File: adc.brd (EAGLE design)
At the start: 20 parts, among them U1 LM4562MAX/NOPB

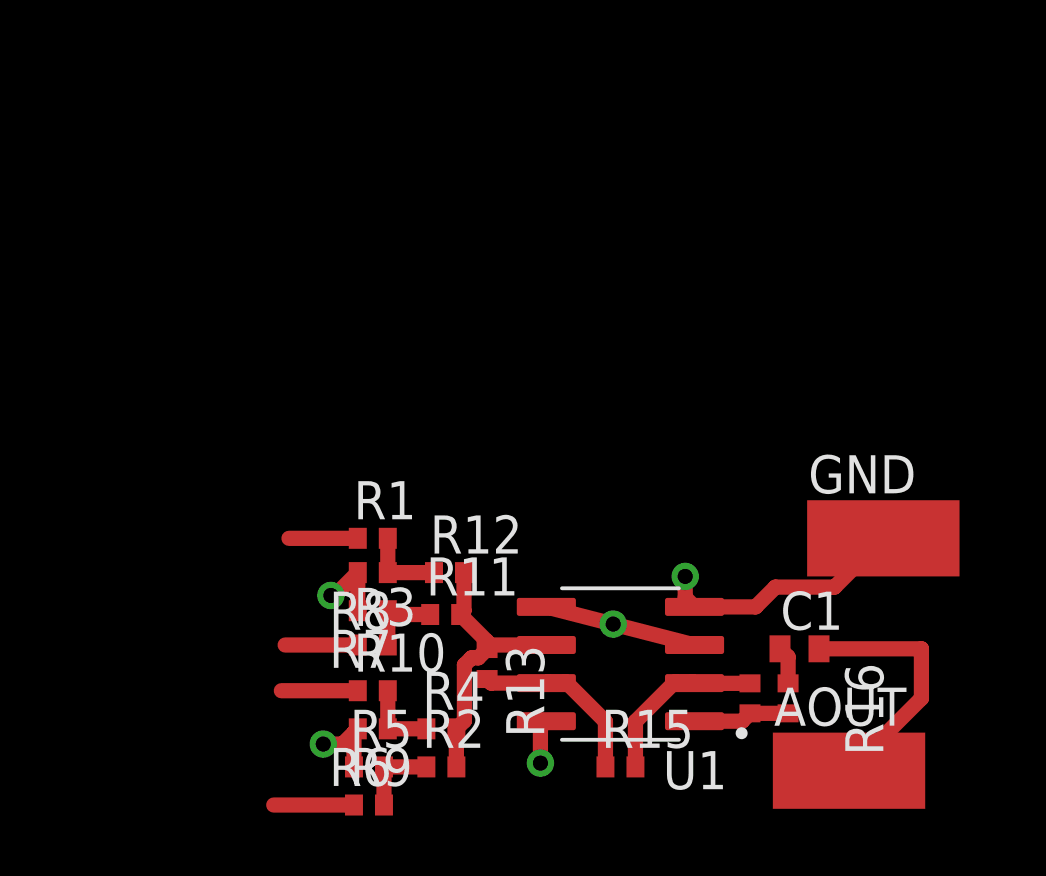
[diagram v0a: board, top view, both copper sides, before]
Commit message: corrections
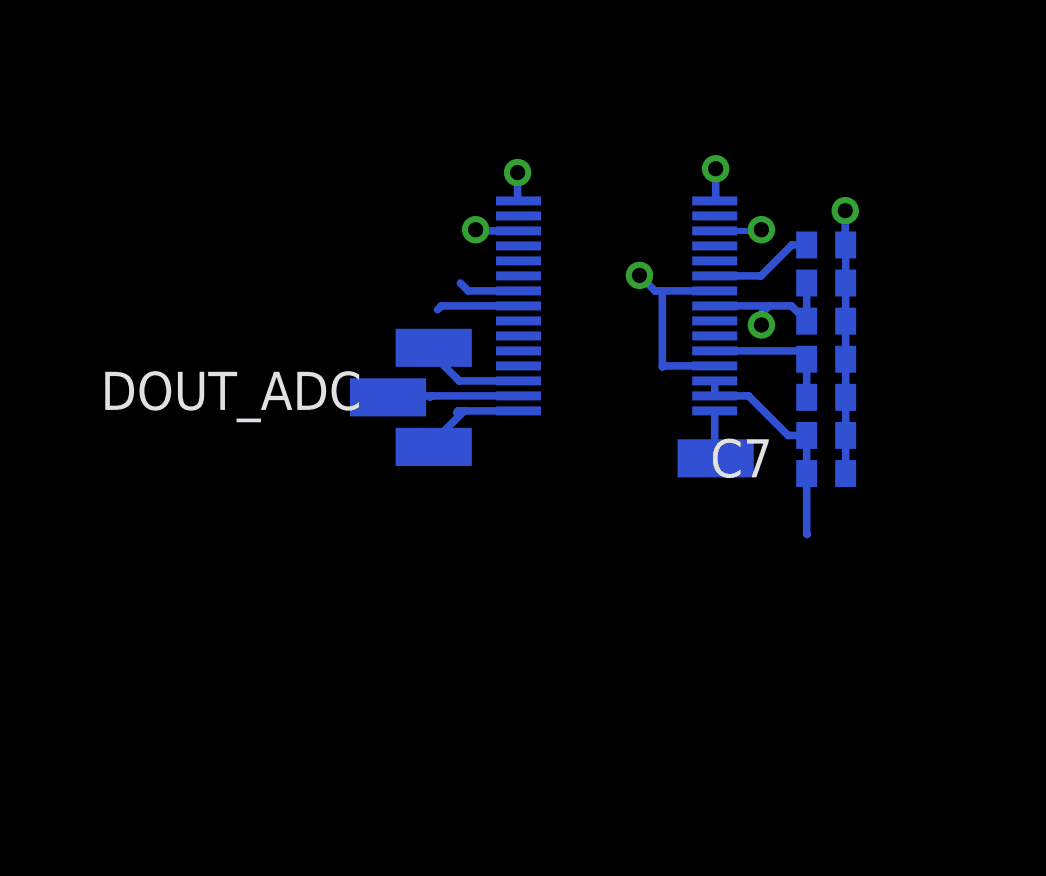
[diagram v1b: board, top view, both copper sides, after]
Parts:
- removed AOUT, GND: (no value), wirepad:SMD2,54-5,08
- removed R1, R10, R3, R5, R6, R7, R8, R9: 5k, rcl:R0402
- removed R11, R12, R13, R14, R15, R2, R4: 20k, rcl:R0402
- removed R16: 1k, rcl:R0402
- removed U1: LM4562MAX/NOPB, LM4562MAX_NOPB:SOIC127P599X175-8N
- added BCK_ADC, CLK_ADC, DOUT_ADC, LRCK_ADC: (no value), wirepad:SMD1,27-2,54
- added C2, C4: 10μF, rcl:C0402
- added C3, C6: 0.1μF, rcl:C0402
- added C5, C7: 1μF, rcl:C0402
- added IC1: PCM1865DBT, PCM1865DBT:TSSOP-30
- C1: value 0.1u -> 0.1μF
- moved C1 7.17 mm to (19.7, 14.7), flipped to the bottom, turned to 180 degrees
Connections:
- removed net AIN0: R9.1
- removed net AIN1: R10.1
- removed net AIN2: R3.1
- removed net AIN3: R1.1
- removed net AOUT: AOUT.1, C1.2
- removed net N$1: C1.1, R16.2
- removed net N$13: R2.1, R5.2, R9.2
- removed net N$14: R11.2, R12.2, R13.1, R2.2, R4.2, U1.6
- removed net N$15: R1.2, R12.1, R8.1
- removed net N$16: R11.1, R3.2, R7.1
- removed net N$17: R10.2, R4.1, R6.1
- removed net N$2: R14.2, R16.1, U1.1
- removed net N$4: R13.2, R15.1, U1.7
- removed net N$5: R14.1, R15.2, U1.2
- removed net VDD: U1.8
- removed net VREF: R5.1, R6.2, R7.2, R8.2, U1.3, U1.5
- new net 3V3A: C3.1, C4.1, IC1.8
- new net 3V3D: C1.1, C2.1, IC1.13, IC1.14
- new net BCK_ADC: BCK_ADC.1, IC1.17
- new net CLK_ADC: CLK_ADC.1, IC1.15
- new net DOUT_ADC: DOUT_ADC.1, IC1.18
- new net LRCK_ADC: IC1.16, LRCK_ADC.1
- new net N$10: C5.1, IC1.6
- new net N$11: C6.1, C7.1, IC1.11
- new net SCL: IC1.24
- new net SDA: IC1.23
- new net VIN1: IC1.1
- new net VIN2: IC1.3
- new net VIN3: IC1.30
- new net VIN4: IC1.28
- net GND: now also C1.2, C2.2, C3.2, C4.2, C5.2, C6.2, C7.2, IC1.12, IC1.7; no longer GND.1, U1.4
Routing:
- net VREF: track 25.1 -> 0.00 mm, vias 3 -> 0
- net GND: track 8.38 -> 23.5 mm, vias 1 -> 2
- net N$14: track 9.50 -> 0.00 mm
- net AOUT: track 8.48 -> 0.00 mm
- net 3V3D: track 0.00 -> 7.42 mm
- net N$4: track 6.08 -> 0.00 mm
- net N$5: track 5.90 -> 0.00 mm
- net 3V3A: track 0.00 -> 5.29 mm, vias 0 -> 1
- net N$11: track 0.00 -> 4.45 mm
- net BCK_ADC: track 0.00 -> 4.44 mm
- net LRCK_ADC: track 0.00 -> 3.71 mm
- net N$10: track 0.00 -> 3.49 mm
- net DOUT_ADC: track 0.00 -> 3.43 mm
- net N$2: track 3.23 -> 0.00 mm
- net SDA: track 0.00 -> 2.75 mm
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
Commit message: updates
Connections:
- net VIN1 renamed IN1L_ADC
- net VIN2 renamed IN2L_ADC
- net VIN3 renamed IN3L_ADC
- net VIN4 renamed IN4L_ADC
- new net IN1R_ADC: IC1.2
- new net IN2R_ADC: IC1.4
- new net IN3R_ADC: IC1.29
- new net IN4R_ADC: IC1.27
- net GND: now also IC1.25
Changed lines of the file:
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@@
 <wire x1="6.604" y1="14.534" x2="6.604" y2="14.351" width="0.254" layer="16"/>
 </signal>
-<signal name="VIN2">
+<signal name="IN2L_ADC">
 <contactref element="IC1" pad="3"/>
 <via x="17.526" y="21.59" extent="1-16" drill="0.508"/>
@@
 <wire x1="17.486" y1="21.55" x2="15.97" y2="21.55" width="0.2032" layer="16"/>
 </signal>
-<signal name="VIN1">
+<signal name="IN1L_ADC">
 <contactref element="IC1" pad="1"/>
 <wire x1="15.97" y1="22.55" x2="16.002" y2="22.582" width="0.254" layer="16"/>
@@
 <wire x1="6.858" y1="19.05" x2="6.731" y2="18.923" width="0.254" layer="16"/>
 </signal>
-<signal name="VIN3">
+<signal name="IN3L_ADC">
 <contactref element="IC1" pad="30"/>
 <wire x1="9.43" y1="22.55" x2="9.398" y2="22.582" width="0.254" layer="16"/>
@@
 <via x="9.398" y="23.495" extent="1-16" drill="0.508"/>
 </signal>
-<signal name="VIN4">
+<signal name="IN4L_ADC">
 <contactref element="IC1" pad="28"/>
 <wire x1="9.43" y1="21.55" x2="8.168" y2="21.55" width="0.254" layer="16"/>
@@
 <wire x1="20.32" y1="22.225" x2="18.161" y2="20.066" width="0.254" layer="2"/>
 <wire x1="18.161" y1="20.066" x2="13.462" y2="20.066" width="0.254" layer="2"/>
+<contactref element="IC1" pad="25"/>
+<wire x1="9.43" y1="20.05" x2="13.462" y2="20.066" width="0" layer="19" extent="16-16"/>
 </signal>
 <signal name="3V3D">
@@
 <via x="17.526" y="18.415" extent="1-16" drill="0.508"/>
 </signal>
+<signal name="IN1R_ADC">
+<contactref element="IC1" pad="2"/>
+</signal>
+<signal name="IN2R_ADC">
+<contactref element="IC1" pad="4"/>
+</signal>
+<signal name="IN3R_ADC">
+<contactref element="IC1" pad="29"/>
+</signal>
+<signal name="IN4R_ADC">
+<contactref element="IC1" pad="27"/>
+</signal>
 </signals>

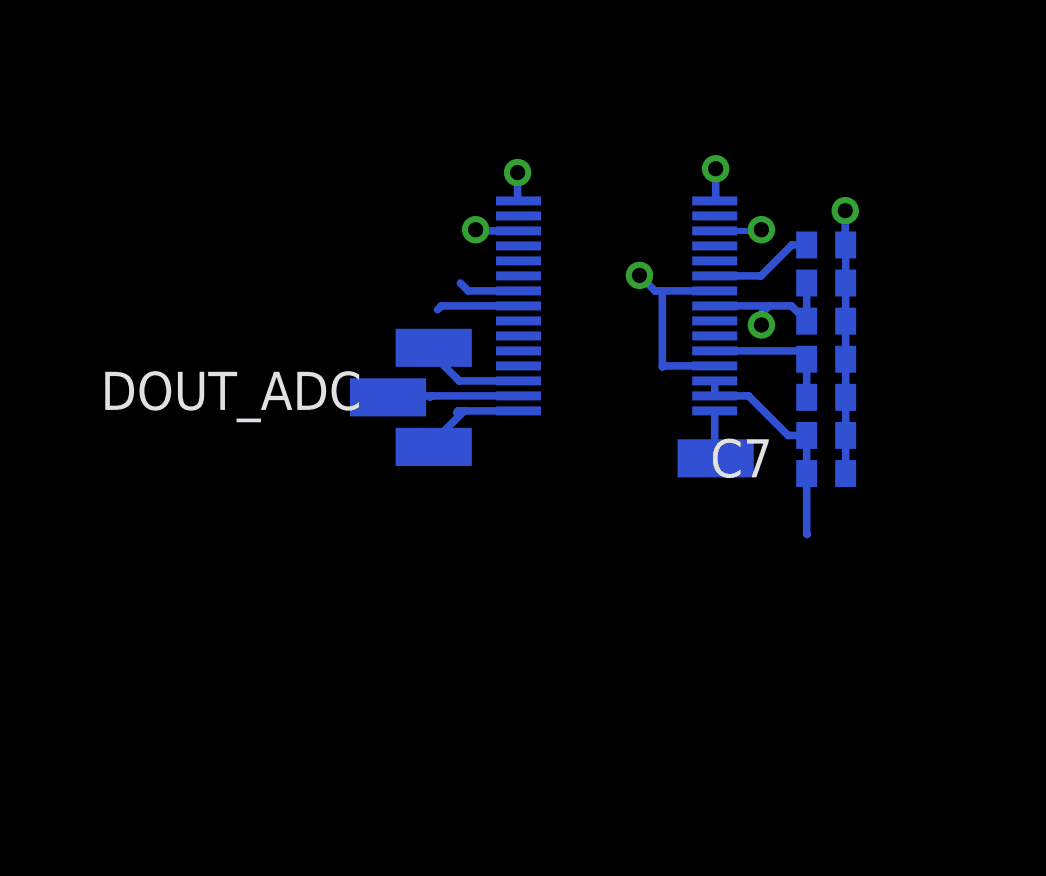
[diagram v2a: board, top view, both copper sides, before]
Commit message: v2 of board finished
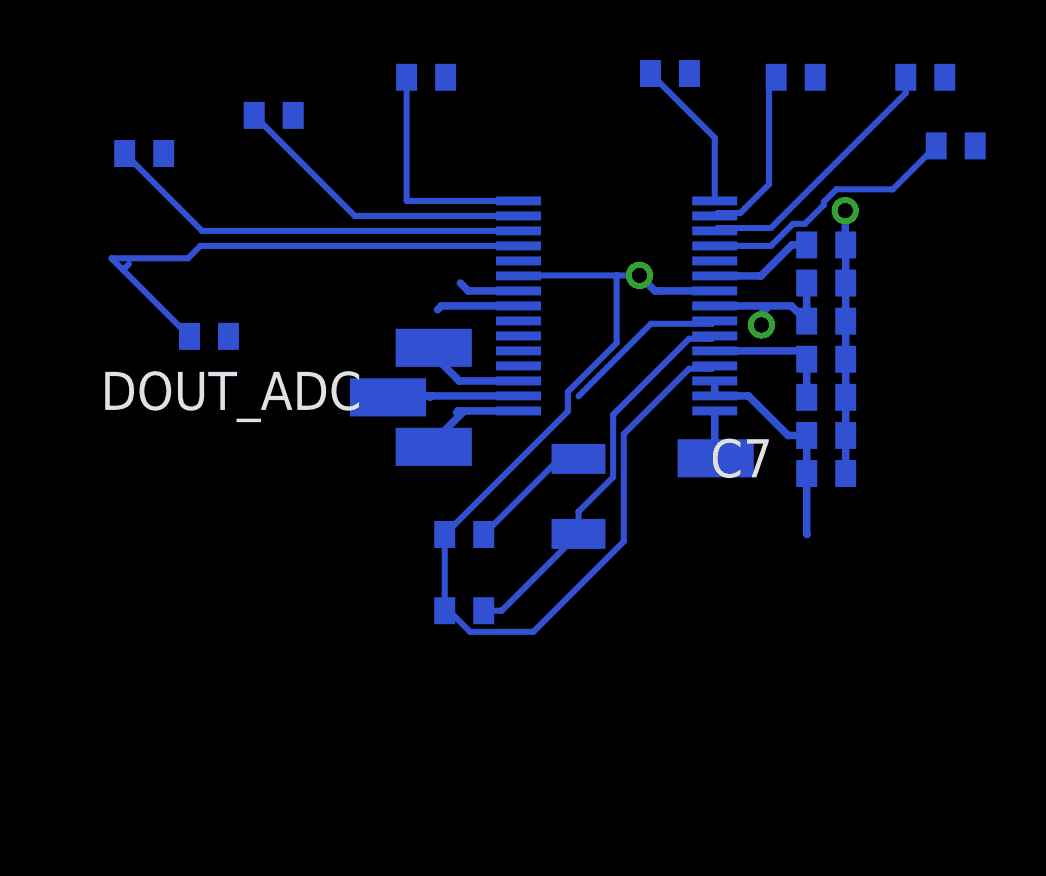
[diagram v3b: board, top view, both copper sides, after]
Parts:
- added C10, C11, C12, C13, C14, C15, C17, C18: 10uF, rcl:C0402
- added C8, C9: 15pF, rcl:C0402
- added Y1: CM7V-T1A-32.768KHZ-12.5PF-100PPM-TB-QC, CM7V-T1A-32.768KHZ-12.5PF-100PPM-TB-QC:XTAL_CM7V-T1A-32.768KHZ-12.5PF-100PPM-TB-QC
- C1, C3, C6: value 0.1μF -> 0.1uF
- C2, C4: value 10μF -> 10uF
- C5, C7: value 1μF -> 1uF
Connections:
- removed net IN1L_ADC: IC1.1
- removed net IN1R_ADC: IC1.2
- removed net IN2L_ADC: IC1.3
- removed net IN2R_ADC: IC1.4
- removed net IN3L_ADC: IC1.30
- removed net IN3R_ADC: IC1.29
- removed net IN4L_ADC: IC1.28
- removed net IN4R_ADC: IC1.27
- new net N$1: C8.1, IC1.9, Y1.2
- new net N$12: C17.2, IC1.28
- new net N$13: C13.2, IC1.27
- new net N$14: C17.1
- new net N$15: C13.1
- new net N$17: C11.1
- new net N$18: C14.1
- new net N$19: C10.1
- new net N$2: C9.1, IC1.10, Y1.1
- new net N$20: C18.1
- new net N$21: C15.2, IC1.30
- new net N$3: C15.1
- new net N$4: C12.1
- new net N$5: C18.2, IC1.1
- new net N$6: C10.2, IC1.2
- new net N$7: C14.2, IC1.3
- new net N$8: C11.2, IC1.4
- new net N$9: C12.2, IC1.29
- net GND: now also C8.2, C9.2
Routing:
- net GND: track 23.5 -> 51.9 mm
- net N$13: track 0.00 -> 17.7 mm
- net N$12: track 0.00 -> 14.2 mm
- net N$2: track 0.00 -> 13.1 mm
- net N$9: track 0.00 -> 10.2 mm
- net N$1: track 0.00 -> 9.14 mm
- net N$8: track 0.00 -> 8.82 mm
- net N$7: track 0.00 -> 8.80 mm
- net N$21: track 0.00 -> 7.85 mm
- net N$6: track 0.00 -> 5.91 mm
- net N$5: track 0.00 -> 5.13 mm
- net IN2L_ADC: track 1.57 -> 0.00 mm, vias 1 -> 0
- net IN4L_ADC: track 1.50 -> 0.00 mm, vias 1 -> 0
- net IN1L_ADC: track 1.09 -> 0.00 mm, vias 1 -> 0
- net IN3L_ADC: track 0.96 -> 0.00 mm, vias 1 -> 0
